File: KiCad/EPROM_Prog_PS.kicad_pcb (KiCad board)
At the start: 2 copper layers, 39 x 56.5 mm, 25 parts, among them J1 13Vdc_In, J2 Prog_EN, J3 Vpp_Vcc_Out, Q1 SST3904, Q2 TM2301GN, U1 LM317L_TO92

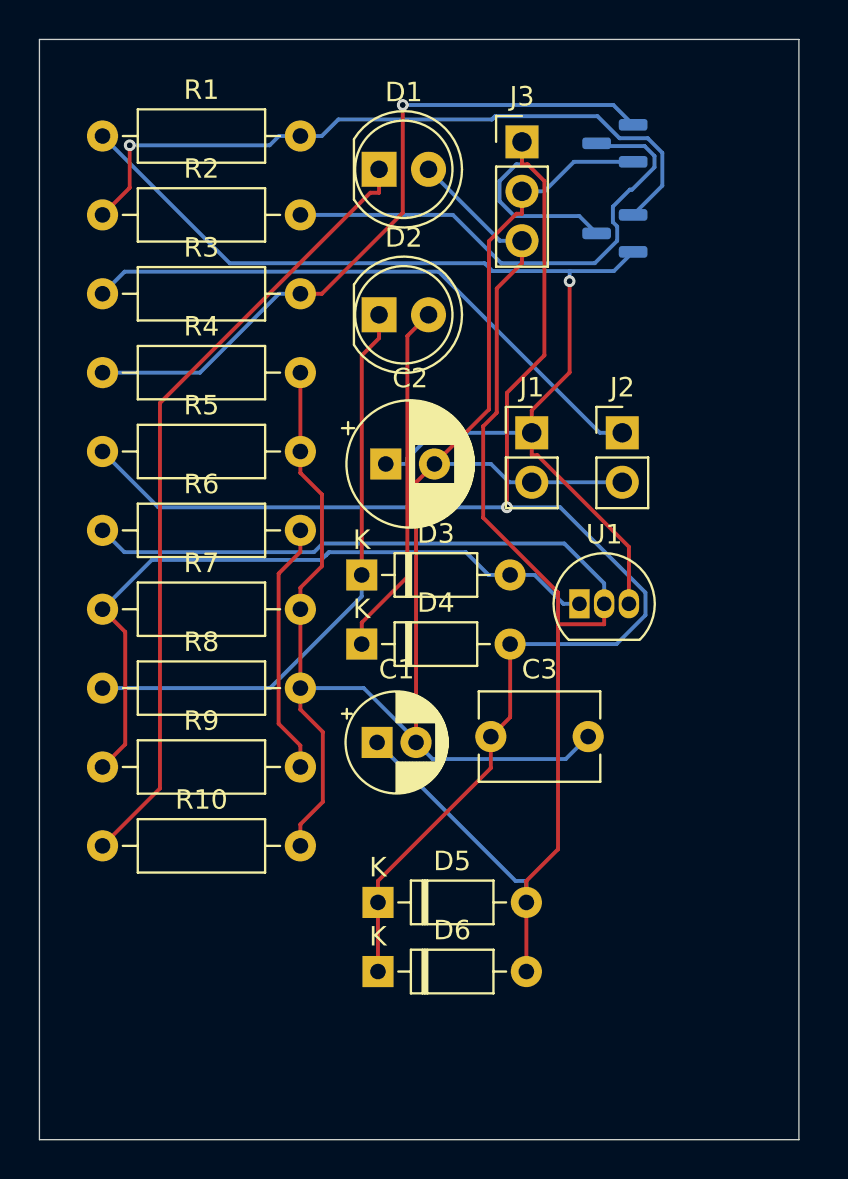
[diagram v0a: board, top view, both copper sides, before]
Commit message: PCB Design
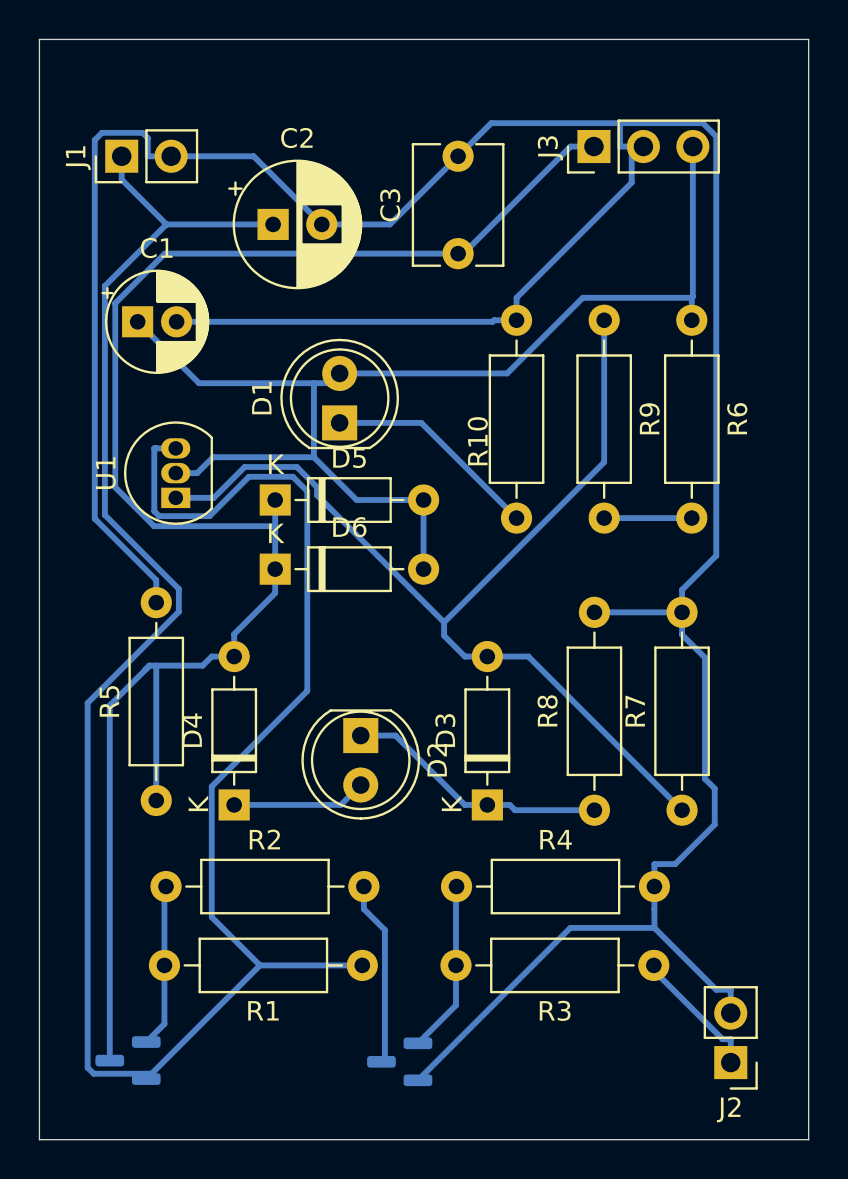
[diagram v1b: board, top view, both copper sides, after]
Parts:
- moved Q2 49.3 mm to (19.6, 67.4)
- moved Q1 48.4 mm to (33.5, 67.5)
- moved R1 44.6 mm to (31.6, 62.5), turned to 180 degrees
- moved R3 44.6 mm to (46.6, 62.5), turned to 180 degrees
- moved R2 34.6 mm to (21.5, 58.5)
- moved R9 34.5 mm to (44.0, 29.4), turned to -90 degrees
- moved J2 32.8 mm to (50.5, 67.5), turned to 180 degrees
- moved R6 32.1 mm to (48.5, 29.4), turned to -90 degrees
- moved R4 32.0 mm to (36.4, 58.5)
- moved R7 31.5 mm to (48.0, 54.6), turned to 90 degrees
- moved R10 27.1 mm to (39.5, 39.6), turned to 90 degrees
- moved R8 26.0 mm to (43.5, 54.6), turned to 90 degrees
- moved J1 25.4 mm to (19.2, 21.0), turned to 90 degrees
- moved C3 24.9 mm to (36.5, 26.0), turned to 90 degrees
- moved C1 24.9 mm to (20.0, 29.5)
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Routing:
- net GND: track 90.1 -> 163.6 mm
- net Net-(J1-Pin_1): track 59.0 -> 115.7 mm, vias 1 -> 0
- net Net-(D1-K): track 40.9 -> 11.1 mm
- net Net-(D1-A): track 90.4 -> 61.8 mm
- net Net-(Q2-G): track 36.9 -> 8.41 mm, vias 1 -> 0
- net Net-(Q1-B): track 36.6 -> 8.87 mm, vias 1 -> 0
- net Net-(J2-Pin_1): track 30.6 -> 6.87 mm
- net Net-(D3-A): track 36.1 -> 53.5 mm
- net Net-(Q1-C): track 26.4 -> 9.52 mm
- net Net-(D2-K): track 30.1 -> 13.6 mm
- net Net-(D2-A): track 18.3 -> 6.92 mm
- net Net-(R6-Pad2): track 13.1 -> 4.50 mm
- net Net-(D4-A): track 88.8 -> 88.2 mm, vias 1 -> 0
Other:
- board size 39 x 56.5 mm -> 39.5 x 56.5 mm
